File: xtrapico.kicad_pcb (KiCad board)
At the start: 2 copper layers, 36.4 x 23.1 mm, 36 parts, among them U2 W25Q128JVS, U3 RP2040, U4 AZ1117R-3_3TRE1, U5 X1321FR-2X20-C43D24, U6 B5819W_C8598, U7 B5819W_C8598, X1 X322512MSB4SI

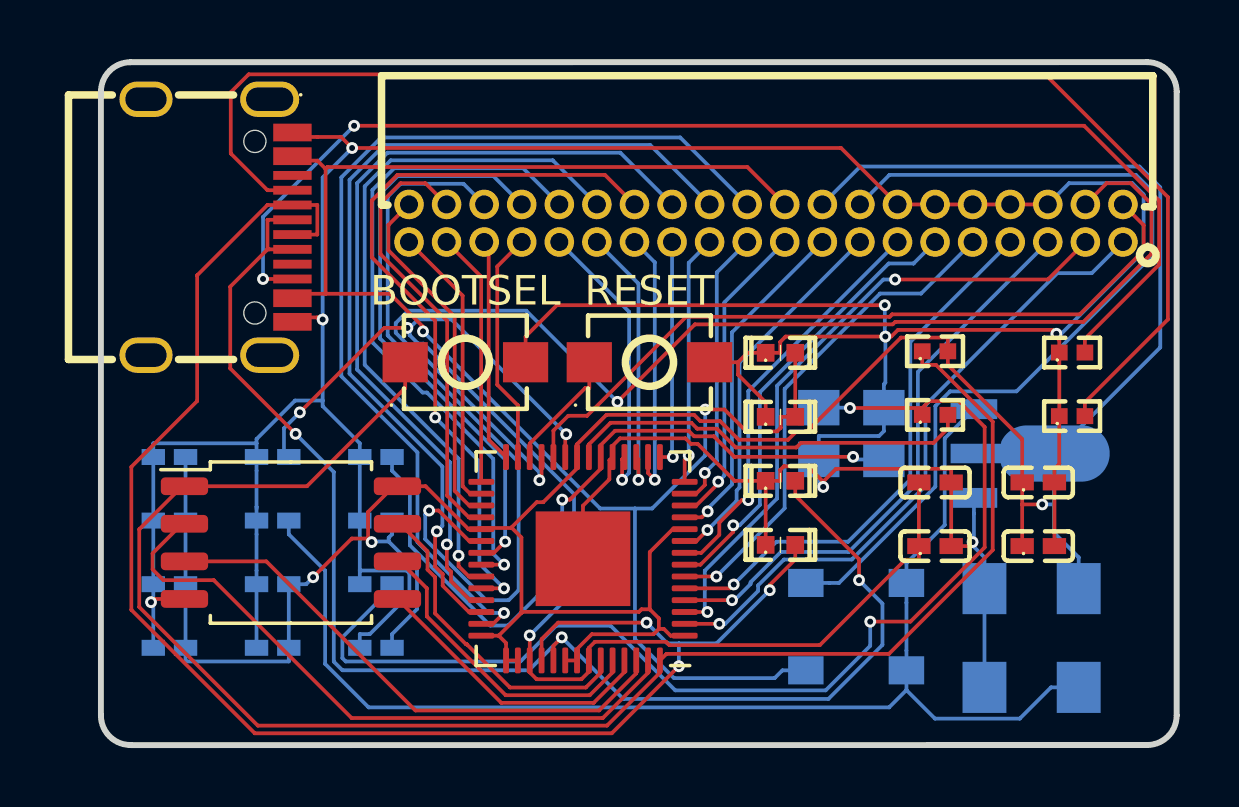
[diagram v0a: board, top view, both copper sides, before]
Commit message: update
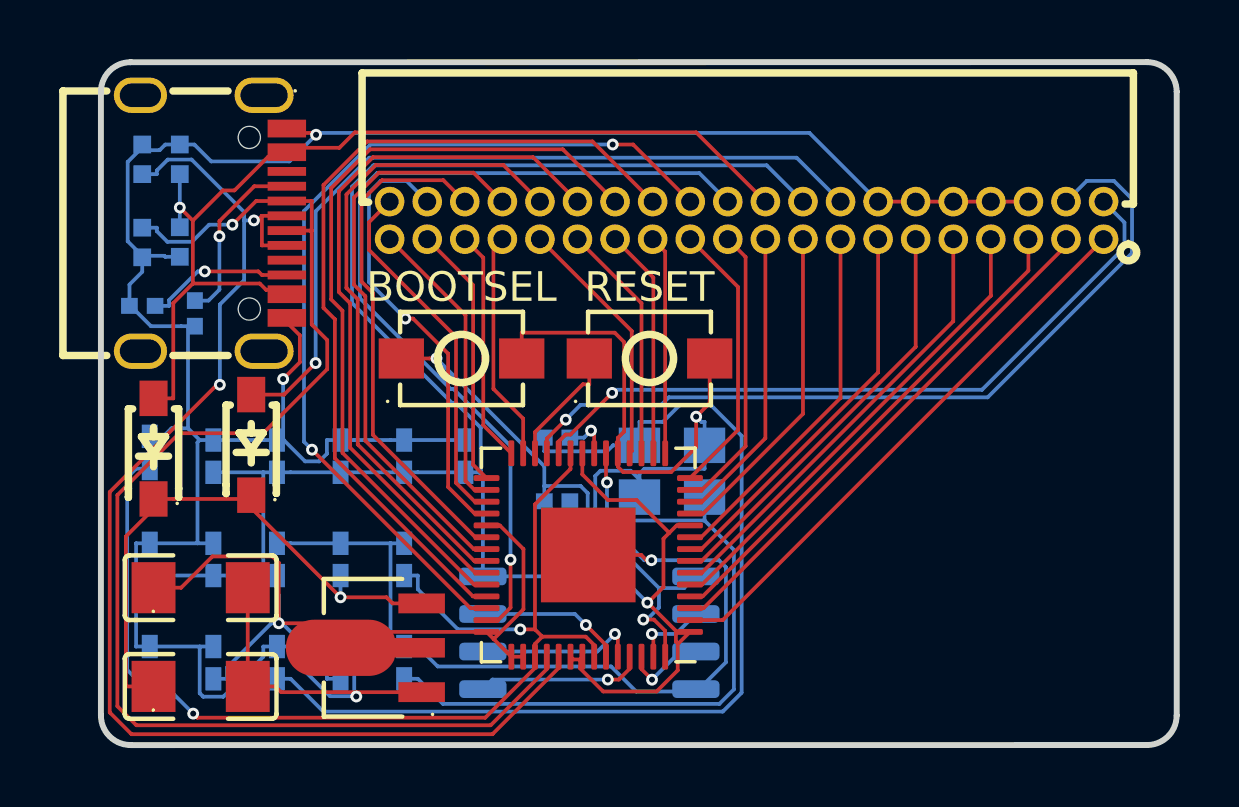
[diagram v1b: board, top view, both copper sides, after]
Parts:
- removed C1, C3: 0402CG300J500NT, JLCPCB:C0402
- removed C10, C11, C12, C13, C15, C16, C17, C18, C2, C5, C6, C7, C8, C9: CL05A106MQ5NUNC, JLCPCB:C0402
- removed C14, C4: CL31A107MQHNNNE, JLCPCB:C1206
- removed D1, D2, D3, D4: 0402ESDA-05N, JLCPCB:D0402-BI
- removed R1, R3: 0402WGF5101TCE, JLCPCB:R0402
- removed R2: 0402WGF1002TCE, JLCPCB:R0402
- removed R4: 0402WGF1001TCE, JLCPCB:R0402
- removed U2: W25Q128JVS, Package_SO:SOIC-8_5.23x5.23mm_P1.27mm
- removed U3: RP2040, Package_DFN_QFN:QFN-56-1EP_7x7mm_P0.4mm_EP3.2x3.2mm
- removed U4: AZ1117R-3_3TRE1, JLCPCB:SOT-89-3_L4.5-W2.5-P1.50-LS4.2-BR
- removed U5: X1321FR-2X20-C43D24, JLCPCB:CONN-TH_40P_X1321FR-2X20-C43D24
- removed U6, U7: B5819W_C8598, JLCPCB:SOD-123_L2.7-W1.6-LS3.7-RD-1
- removed X1: X322512MSB4SI, JLCPCB:OSC-SMD_4P-L3.2-W2.5-BL
- added XTRAPI_C1: 0402CG300J500NT, JLCPCB:C0402, B.Cu at (25.1, 34.8)
- added XTRAPI_C10: CL05A106MQ5NUNC, JLCPCB:C0402, B.Cu at (20.8, 31.3)
- added XTRAPI_C11: CL05A106MQ5NUNC, JLCPCB:C0402, B.Cu at (18.7, 31.3)
- added XTRAPI_C12: CL05A106MQ5NUNC, JLCPCB:C0402, B.Cu at (16.5, 31.3)
- added XTRAPI_C13: CL05A106MQ5NUNC, JLCPCB:C0402, B.Cu at (27.2, 27.8)
- added XTRAPI_C14: CL31A107MQHNNNE, JLCPCB:C1206, F.Cu at (18.2, 35.6)
- added XTRAPI_C15: CL05A106MQ5NUNC, JLCPCB:C0402, B.Cu at (25.1, 27.8)
- added XTRAPI_C16: CL05A106MQ5NUNC, JLCPCB:C0402, B.Cu at (23.0, 27.8)
- added XTRAPI_C17: CL05A106MQ5NUNC, JLCPCB:C0402, B.Cu at (20.8, 27.8)
- added XTRAPI_C18: CL05A106MQ5NUNC, JLCPCB:C0402, B.Cu at (18.7, 27.8)
- added XTRAPI_C2: CL05A106MQ5NUNC, JLCPCB:C0402, B.Cu at (23.0, 34.8)
- added XTRAPI_C3: 0402CG300J500NT, JLCPCB:C0402, B.Cu at (20.8, 34.8)
- added XTRAPI_C4: CL31A107MQHNNNE, JLCPCB:C1206, F.Cu at (18.2, 32.3)
- added XTRAPI_C5: CL05A106MQ5NUNC, JLCPCB:C0402, B.Cu at (18.7, 34.8)
- added XTRAPI_C6: CL05A106MQ5NUNC, JLCPCB:C0402, B.Cu at (16.5, 34.8)
- added XTRAPI_C7: CL05A106MQ5NUNC, JLCPCB:C0402, B.Cu at (16.5, 27.7)
- added XTRAPI_C8: CL05A106MQ5NUNC, JLCPCB:C0402, B.Cu at (25.1, 31.3)
- added XTRAPI_C9: CL05A106MQ5NUNC, JLCPCB:C0402, B.Cu at (23.0, 31.3)
- added XTRAPI_R2: 0402WGF1002TCE, JLCPCB:R0402, B.Cu at (30.3, 29.3)
- added XTRAPI_R4: 0402WGF1001TCE, JLCPCB:R0402, B.Cu at (30.3, 27.2)
- added XTRAPI_U2: W25Q128JVS, Package_SO:SOIC-8_5.23x5.23mm_P1.27mm, B.Cu at (31.4, 33.8)
- added XTRAPI_U3: RP2040, Package_DFN_QFN:QFN-56-1EP_7x7mm_P0.4mm_EP3.2x3.2mm, F.Cu at (31.3, 31.2)
- added XTRAPI_U4: AZ1117R-3_3TRE1, JLCPCB:SOT-89-3_L4.5-W2.5-P1.50-LS4.2-BR, F.Cu at (24.3, 34.3)
- added XTRAPI_U6: B5819W_C8598, JLCPCB:SOD-123_L2.7-W1.6-LS3.7-RD-1, F.Cu at (19.9, 27.4)
- added XTRAPI_U7: B5819W_C8598, JLCPCB:SOD-123_L2.7-W1.6-LS3.7-RD-1, F.Cu at (16.6, 27.6)
- added XTRAPI_X1: X322512MSB4SI, JLCPCB:OSC-SMD_4P-L3.2-W2.5-BL, B.Cu at (34.2, 28.3)
- added XTRA_D1: 0402ESDA-05N, JLCPCB:D0402-BI, B.Cu at (17.5, 20.6)
- added XTRA_D2: 0402ESDA-05N, JLCPCB:D0402-BI, B.Cu at (17.5, 17.8)
- added XTRA_D3: 0402ESDA-05N, JLCPCB:D0402-BI, B.Cu at (16.3, 17.8)
- added XTRA_D4: 0402ESDA-05N, JLCPCB:D0402-BI, B.Cu at (16.3, 20.6)
- added XTRA_R1: 0402WGF5101TCE, JLCPCB:R0402, B.Cu at (16.3, 22.7)
- added XTRA_R3: 0402WGF5101TCE, JLCPCB:R0402, B.Cu at (18.0, 23.0)
- added XTRA_U5: X1321FR-2X20-C43D24, JLCPCB:CONN-TH_40P_X1321FR-2X20-C43D24, F.Cu at (36.7, 19.8)
- moved XTRA_J1 0.23 mm to (18.7, 19.9)
- moved XTRA_SW_BOOTSEL1 0.18 mm to (27.0, 24.5)
- moved XTRA_SW_RESET1 0.13 mm to (33.4, 24.5)
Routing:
- net Net-(U4-INPUT): track 43.0 -> 0.00 mm
- net Net-(XTRA_J1-CC1): track 46.9 -> 6.07 mm, vias 0 -> 1
- net Net-(X1-OSC2): track 39.4 -> 0.00 mm, vias 2 -> 0
- net /BOOTSEL: track 55.7 -> 17.8 mm, vias 0 -> 2
- net Net-(XTRA_J1-CC2): track 41.9 -> 5.10 mm, vias 2 -> 1
- net Net-(XTRAPI_X1-OSC2): track 0.00 -> 33.8 mm
- net Net-(U3-XIN): track 25.4 -> 0.00 mm, vias 2 -> 0
- net Net-(XTRAPI_U3-XIN): track 0.00 -> 24.0 mm, vias 0 -> 1
- net /VBUS: track 58.3 -> 34.7 mm, vias 2 -> 1
- net Net-(U2-DO(IO1)): track 21.9 -> 0.00 mm
- net Net-(XTRAPI_U4-INPUT): track 0.00 -> 19.3 mm, vias 0 -> 1
- net Net-(U2-IO2): track 18.3 -> 0.00 mm
- net /SWD: track 41.8 -> 27.5 mm, vias 2 -> 1
- net Net-(U3-XOUT): track 13.9 -> 0.00 mm
- net Net-(U2-IO3): track 10.9 -> 0.00 mm
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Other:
- board text added: "xtrapico small footprint RP2040 impl"
- board text removed: "xtrapico / small footprint RP2040 impl"
